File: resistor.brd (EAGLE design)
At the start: 10.2 x 39.5 mm, 3 parts

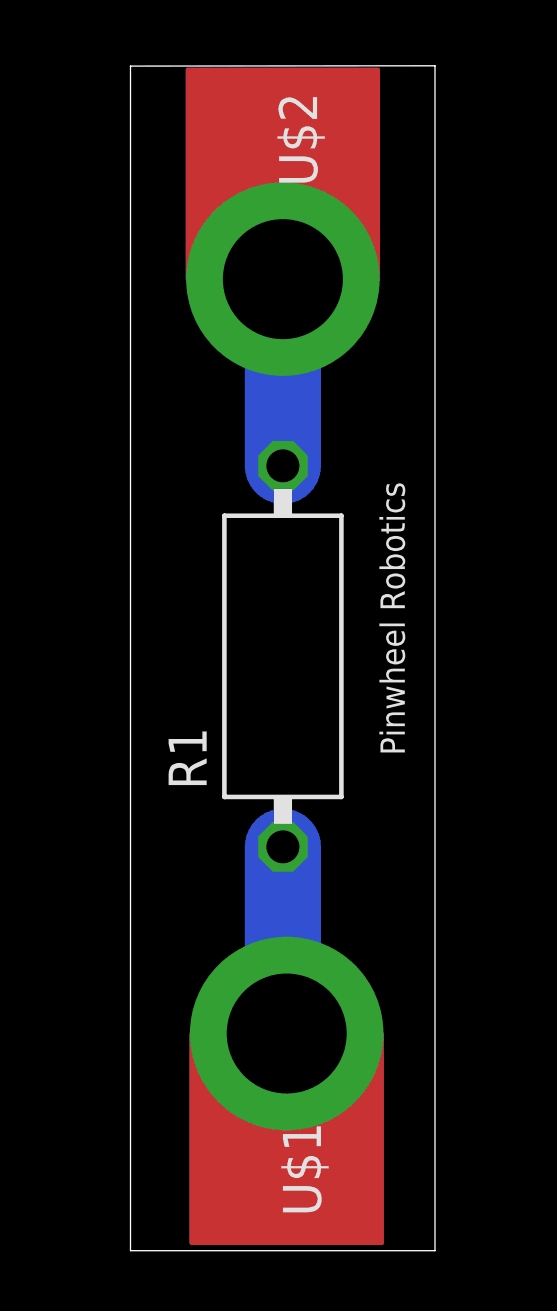
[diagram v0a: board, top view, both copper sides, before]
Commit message: New Updates
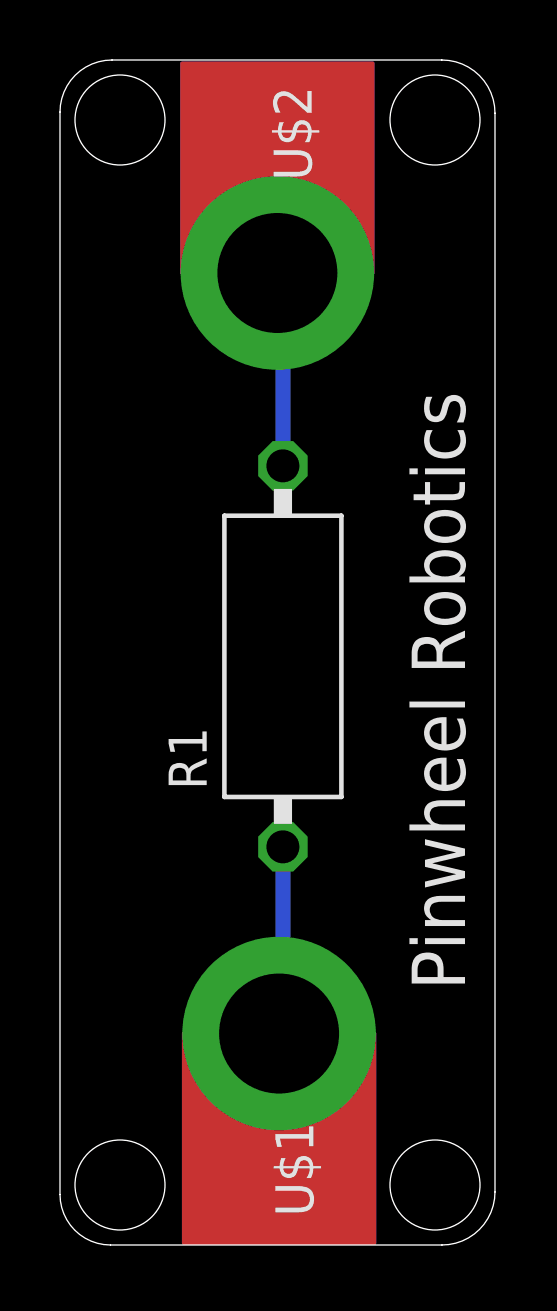
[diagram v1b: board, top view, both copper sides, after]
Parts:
- moved U$2 0.28 mm to (11.2, 36.4)
- moved U$1 0.25 mm to (11.3, 11.0)
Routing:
- net N$1: track 7.11 -> 6.25 mm
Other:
- board size 10.2 x 39.5 mm -> 14.5 x 39.5 mm
- board text added: "care@Pinwheel.in"
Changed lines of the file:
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@@
 <setting verticaltext="up"/>
 </settings>
-<grid distance="50" unitdist="mil" unit="mm" style="lines" multiple="1" display="yes" altdistance="5" altunitdist="mil" altunit="mm"/>
+<grid distance="0.5" unitdist="mm" unit="mm" style="lines" multiple="1" display="yes" altdistance="5" altunitdist="mil" altunit="mm"/>
 <layers>
 <layer number="1" name="Top" color="4" fill="1" visible="yes" active="yes"/>
@@
 <layer number="43" name="vRestrict" color="2" fill="10" visible="yes" active="yes"/>
 <layer number="44" name="Drills" color="7" fill="1" visible="no" active="yes"/>
-<layer number="45" name="Holes" color="7" fill="1" visible="no" active="yes"/>
+<layer number="45" name="Holes" color="7" fill="1" visible="yes" active="yes"/>
 <layer number="46" name="Milling" color="3" fill="1" visible="no" active="yes"/>
 <layer number="47" name="Measures" color="7" fill="1" visible="no" active="yes"/>
@@
 <board>
 <plain>
-<wire x1="6.35" y1="3.81" x2="16.5" y2="3.81" width="0" layer="20"/>
-<wire x1="16.5" y1="3.81" x2="16.5" y2="43.307" width="0" layer="20"/>
-<wire x1="16.5" y1="43.307" x2="6.35" y2="43.297" width="0" layer="20"/>
-<wire x1="6.35" y1="43.297" x2="6.35" y2="3.81" width="0" layer="20"/>
-<text x="15.494" y="20.32" size="0.8128" layer="21" rot="R90">Pinwheel Robotics </text>
+<wire x1="4" y1="41.7659" x2="4" y2="5.683746875" width="0" layer="20"/>
+<wire x1="4" y1="5.683746875" x2="5.683746875" y2="4" width="0" layer="20" curve="90"/>
+<wire x1="5.683746875" y1="4" x2="16.731853125" y2="4" width="0" layer="20"/>
+<wire x1="16.731853125" y1="4" x2="18.5" y2="5.768146875" width="0" layer="20" curve="90"/>
+<wire x1="18.5" y1="5.768146875" x2="18.5" y2="41.728584375" width="0" layer="20"/>
+<wire x1="18.5" y1="41.728584375" x2="16.728584375" y2="43.5" width="0" layer="20" curve="90"/>
+<wire x1="16.728584375" y1="43.5" x2="5.7341" y2="43.5" width="0" layer="20"/>
+<wire x1="5.7341" y1="43.5" x2="4" y2="41.7659" width="0" layer="20" curve="90"/>
+<hole x="6" y="41.5" drill="3"/>
+<hole x="16.5" y="41.5" drill="3"/>
+<hole x="6" y="6" drill="3"/>
+<hole x="16.5" y="6" drill="3"/>
+<text x="17.5" y="12.5" size="1.778" layer="21" rot="R90">Pinwheel Robotics</text>
+<text x="6.858" y="34.036" size="1.778" layer="22" rot="MR270">care@Pinwheel.in</text>
 </plain>
 <attributes>
@@
 <attribute name="VALUE" x="12.065" y="19.177" size="1.27" layer="27" ratio="10" rot="R90"/>
 </element>
-<element name="U$2" library="microbit" package="MICROBIT_PAD" value="MICROBIT_PAD" x="11.43" y="36.195" smashed="yes" rot="R180">
-<attribute name="NAME" x="11.303" y="42.418" size="1.27" layer="21" rot="R270"/>
+<element name="U$2" library="microbit" package="MICROBIT_PAD" value="MICROBIT_PAD" x="11.246" y="36.4" smashed="yes" rot="R180">
+<attribute name="NAME" x="11.119" y="42.623" size="1.27" layer="21" rot="R270"/>
 </element>
-<element name="U$1" library="microbit" package="MICROBIT_PAD" value="MICROBIT_PAD" x="11.557" y="11.049" smashed="yes">
-<attribute name="NAME" x="12.7" y="4.953" size="1.27" layer="21" rot="R90"/>
+<element name="U$1" library="microbit" package="MICROBIT_PAD" value="MICROBIT_PAD" x="11.303" y="11.049" smashed="yes">
+<attribute name="NAME" x="12.446" y="4.953" size="1.27" layer="21" rot="R90"/>
 </element>
 </elements>
@@
 <contactref element="R1" pad="1"/>
 <contactref element="U$1" pad="PAD"/>
-<wire x1="11.43" y1="17.272" x2="11.43" y2="10.16" width="2.54" layer="16"/>
-<wire x1="11.43" y1="10.16" x2="11.557" y2="11.049" width="0" layer="19" extent="16-16"/>
+<wire x1="11.43" y1="17.272" x2="11.43" y2="11.35560625" width="0.508" layer="16"/>
+<wire x1="11.43" y1="11.35560625" x2="11.303" y2="11.049" width="0.508" layer="16" curve="-45"/>
 </signal>
 <signal name="N$2">
 <contactref element="U$2" pad="PAD"/>
 <contactref element="R1" pad="2"/>
-<wire x1="11.43" y1="36.195" x2="11.43" y2="29.972" width="2.54" layer="16"/>
+<wire x1="11.43" y1="29.972" x2="11.43" y2="35.7228625" width="0.508" layer="16"/>
+<wire x1="11.43" y1="35.7228625" x2="11.246" y2="36.4" width="0.508" layer="16" curve="45"/>
 </signal>
 </signals>
